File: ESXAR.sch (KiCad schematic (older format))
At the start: 45 parts, among them P1 ANALOG, P10 USB_A, P11 USB_B, P12 SERVO/INPUT, P13 ANALOG, P16 BREADBOARD_POWER, P17 SENSOR, P18 EXTIO, P19 UNIVERSAL, P2 BREADBOARD, P20 UNIVERSAL, P3 PROGRAM, P4 OPAMP EX, P5 MODEJP, P6 VCCJP, P7 GNDJP, P8 SCREW, SW1 RESET, U1 ESP-WROOM-02, U2 NJM4556A, U3 AUDIO_JACK, U5 TLP222A, U6 Mini360

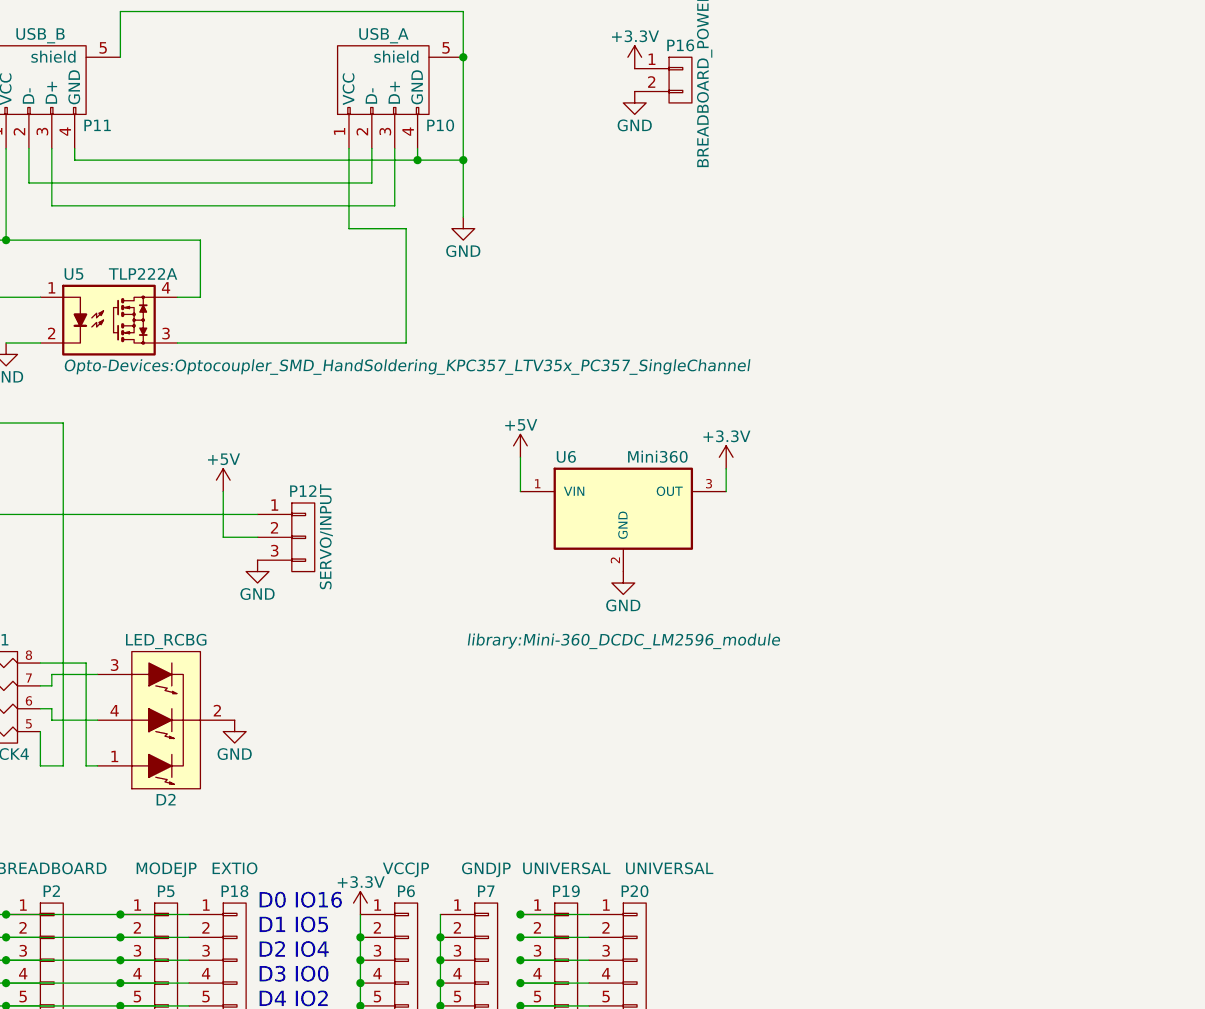
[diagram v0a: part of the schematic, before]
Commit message: Ver 20160804 Layout Change.
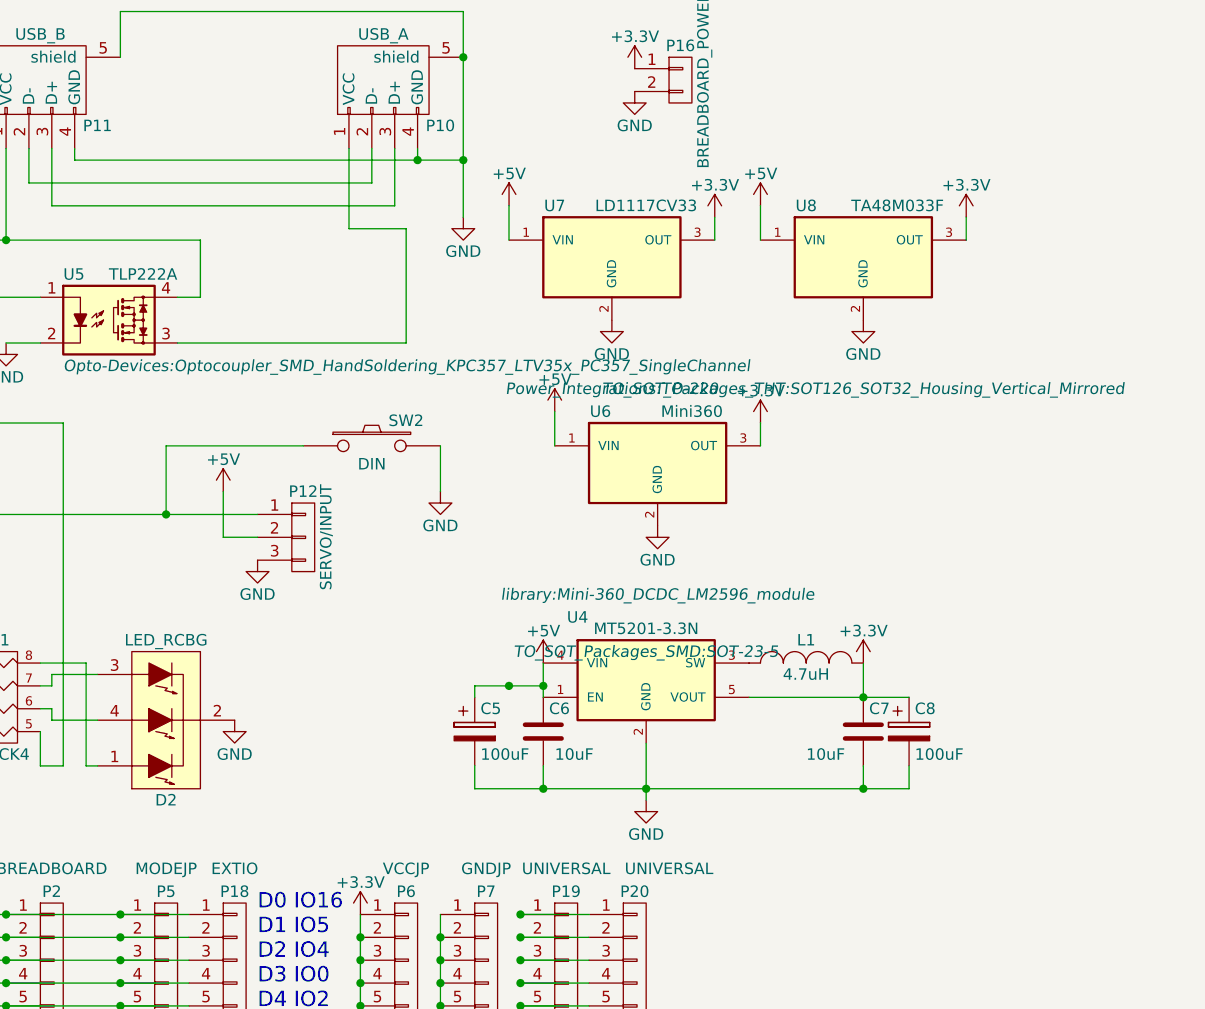
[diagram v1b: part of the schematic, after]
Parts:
- added C5, C8: 100uF, Capacitors_ThroughHole:C_Radial_D6.3_L11.2_P2.5, symbol CP
- added C6, C7: 10uF, library:C_1206_HandSoldering_Small, symbol C
- added L1: 4.7uH, library:C_1206_HandSoldering_Small, symbol INDUCTOR_SMALL
- added SW2: DIN, Buttons_Switches_ThroughHole:SW_PUSH_SMALL, symbol SW_PUSH
- added U4: MT5201-3.3N, TO_SOT_Packages_SMD:SOT-23-5, symbol MT5201-3.3N
- added U7: LD1117CV33, Power_Integrations:TO-220, symbol LT1129MPST-3.3
- added U8: TA48M033F, TO_SOT_Packages_THT:SOT126_SOT32_Housing_Vertical_Mirrored, symbol LT1129MPST-3.3
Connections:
- net +3V3: now also C7.1, C8.1, L1.2, U4.5 (VOUT), U7.3 (OUT), U8.3 (OUT)
- net +5V: now also C5.1, C6.1, U4.1 (EN), U4.4 (VIN), U7.1 (VIN), U8.1 (VIN)
- net GND: now also C5.2, C6.2, C7.2, C8.2, SW2.2, U4.2 (GND), U7.2 (GND), U8.2 (GND)
- net at P12.1 (P1), P18.2 (P2), P2.2 (P2)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: now also SW2.1
- new net: L1.1, U4.3 (SW)
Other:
- moved on the sheet: U6

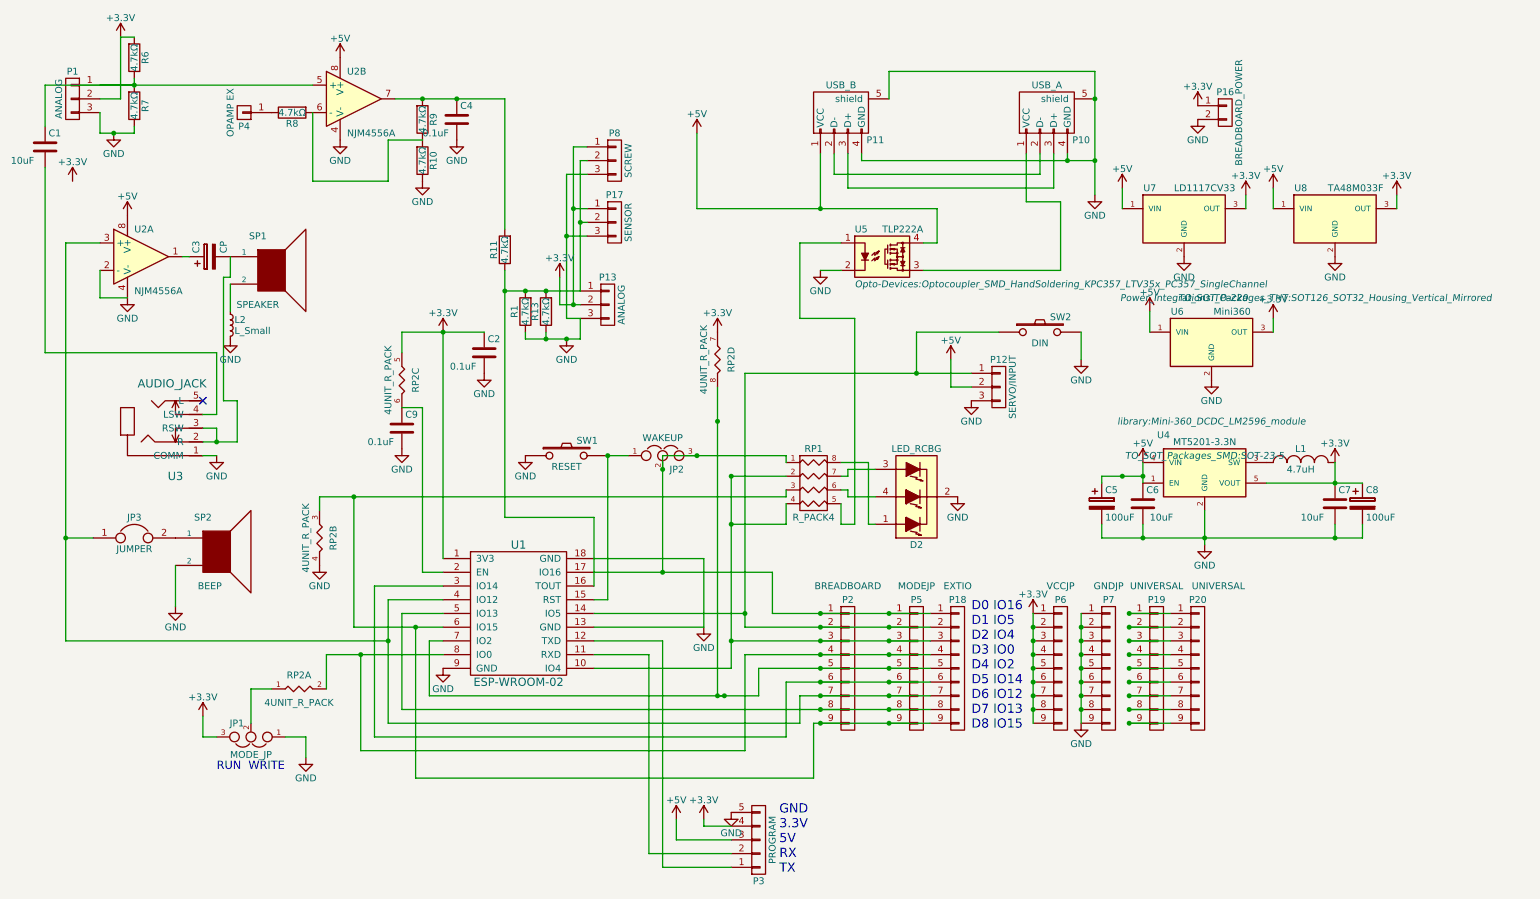
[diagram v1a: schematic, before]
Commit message: Ver.20170816  and documents
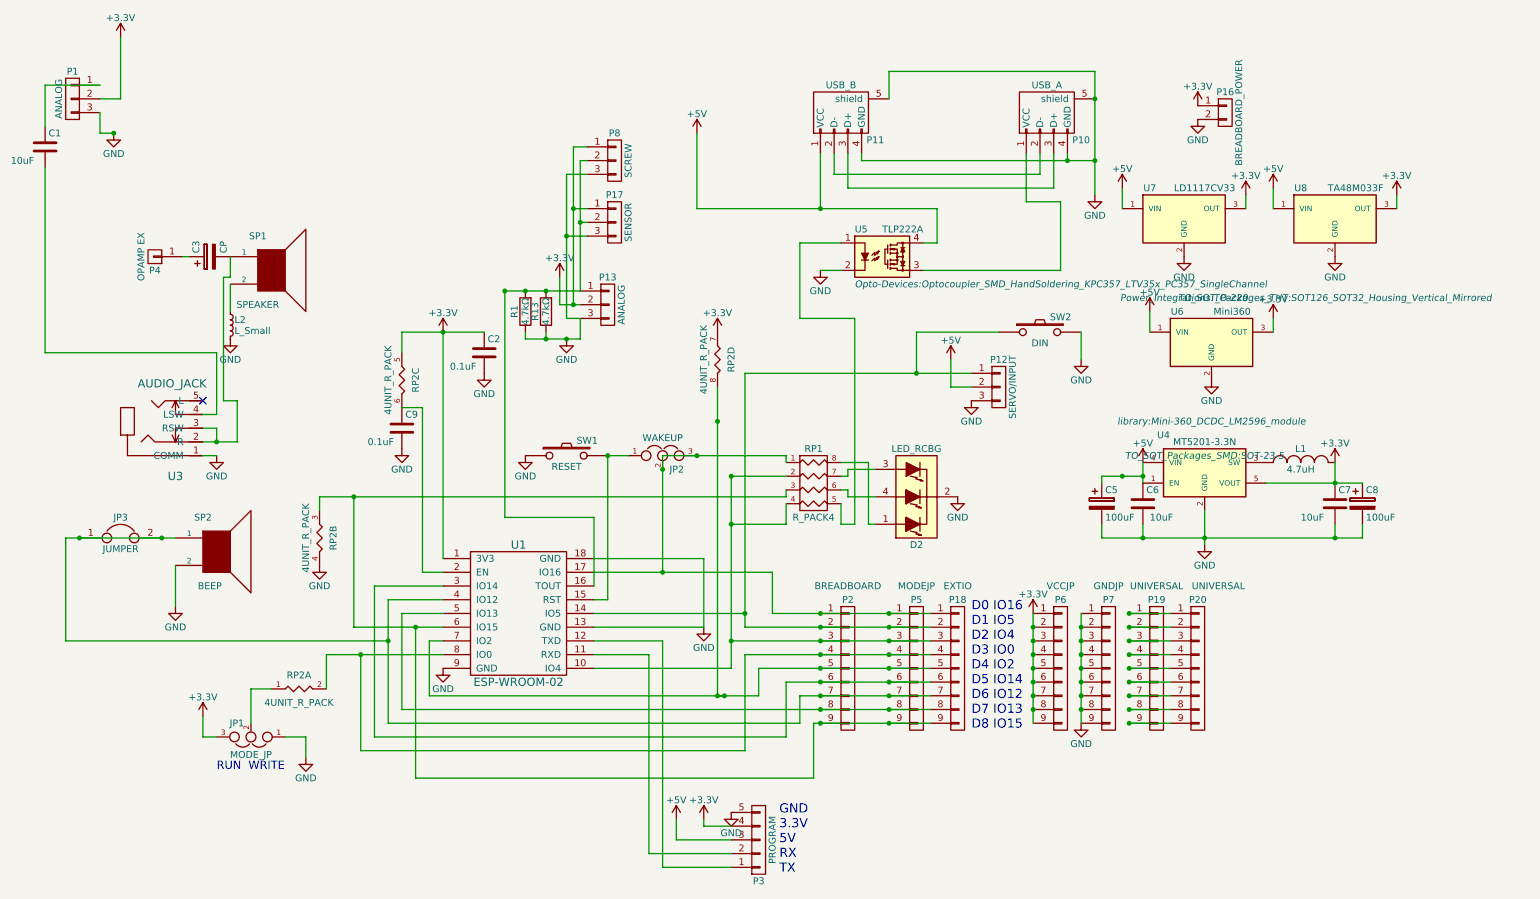
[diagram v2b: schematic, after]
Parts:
- removed C4: 0.1uF, Capacitors_ThroughHole:C_Disc_D3_P2.5, symbol C
- removed R10, R11, R6, R7, R8, R9: 4.7kΩ, Discret:R1, symbol R
- removed U2: NJM4556A, Housings_DIP:DIP-8_W7.62mm, symbol LM358N
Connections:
- net at JP3.1, P18.7 (P7), P2.7 (P7)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: now also JP3.2, SP2.1
- net at C3.1: now also P4.1 (P1)
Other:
- moved on the sheet: JP3, P4
